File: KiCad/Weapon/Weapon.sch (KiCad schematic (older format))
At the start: 29 parts, among them IC1 ATMEGA328-P, J1 MICRO_USB, P1 2P_CGRID_M, P2 USB-TTL, P3 2P_CGRID_M, Q1 NPN, U1 MCP73831, U2 RFID-RC522, U3 LM1084IT-3.3/NOPB, X1 16MHz

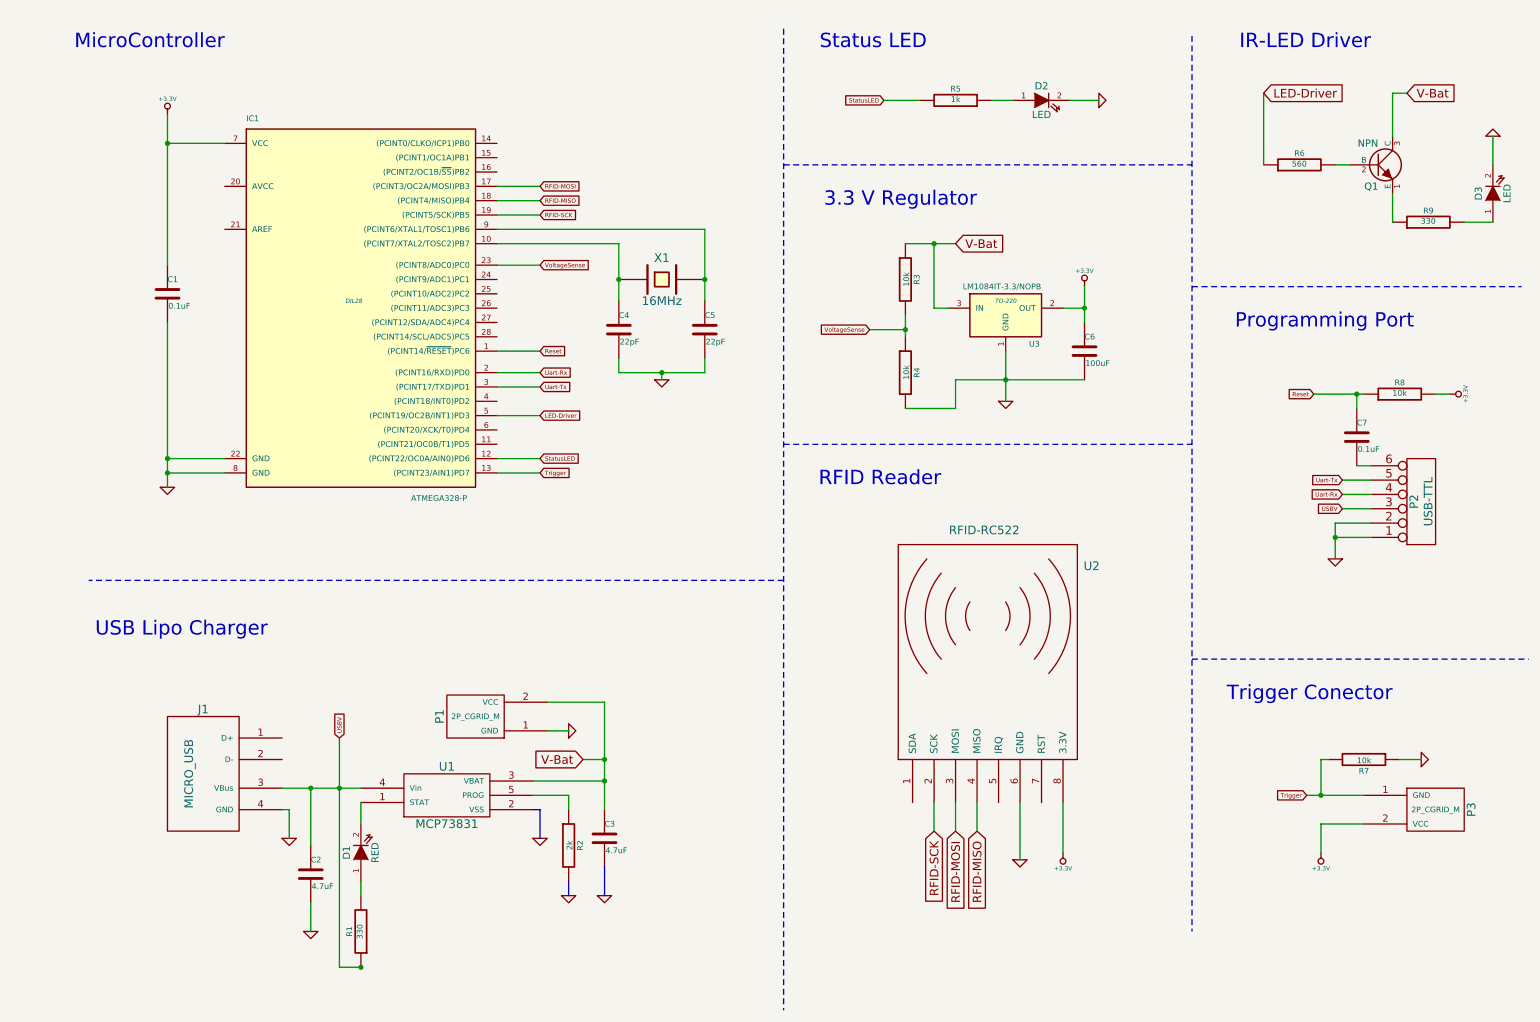
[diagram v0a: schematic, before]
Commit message: Revert "Revert "3/29 KiCad Updates""
This reverts commit 46467126b97e8d3ee2ff82587e11af580e6d6854.
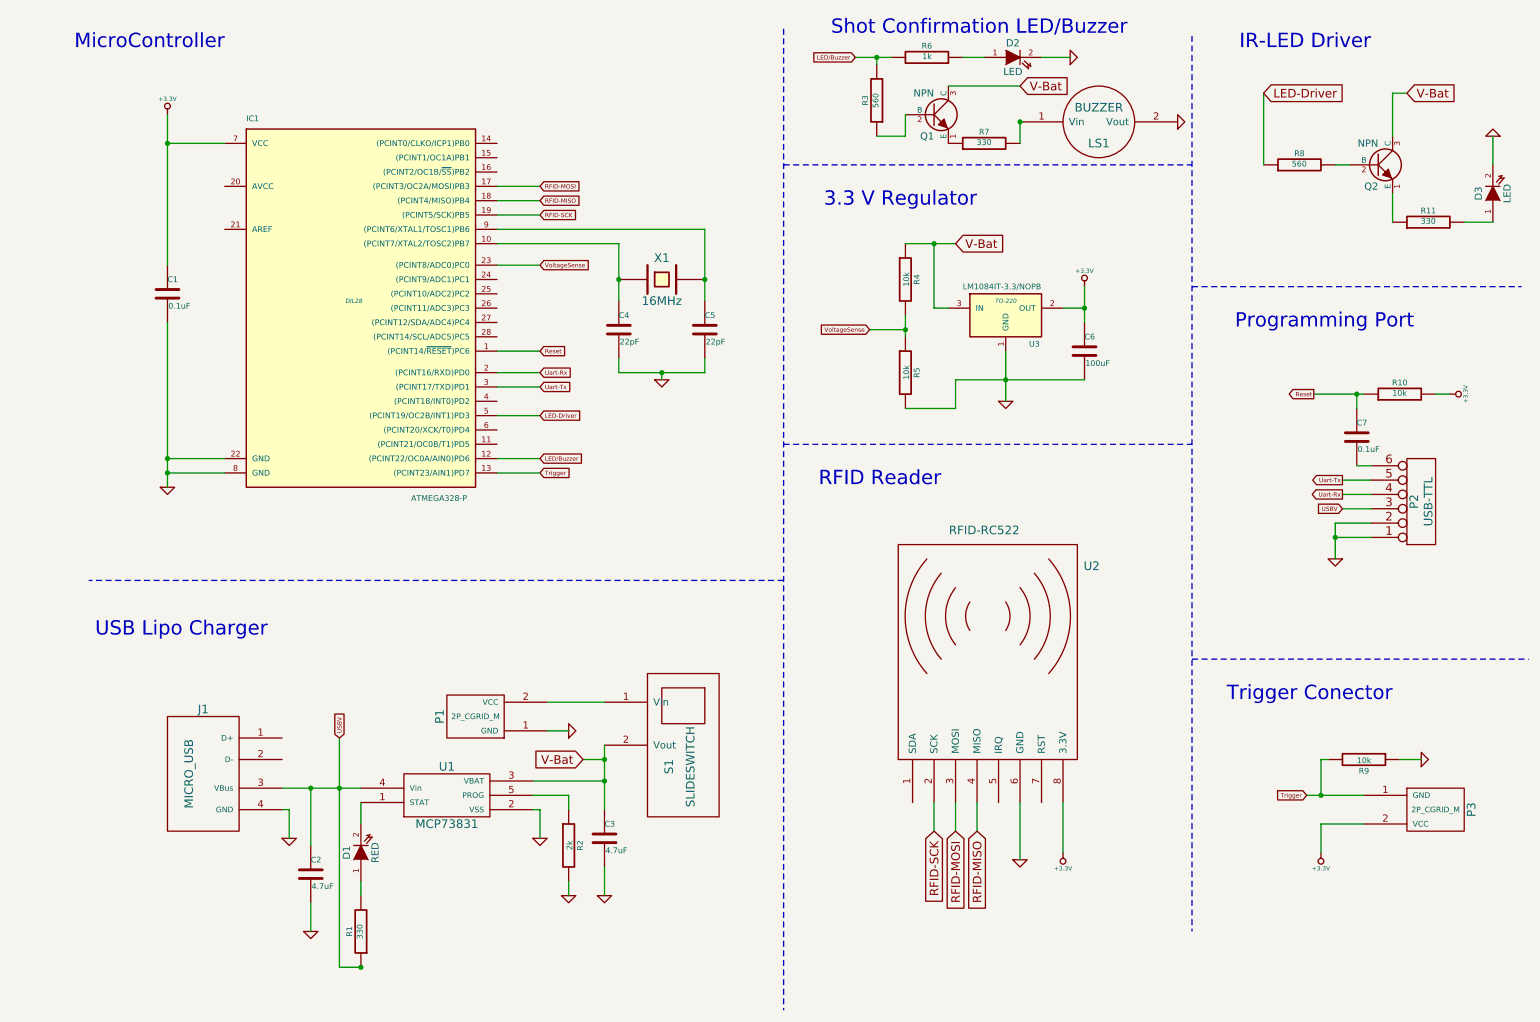
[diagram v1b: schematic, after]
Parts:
- added LS1: BUZZER, symbol BUZZER
- added Q1: NPN, ~, symbol NPN
- added R3: 560, ~, symbol R
- added R7: 330, ~, symbol R
- added S1: SLIDESWITCH, symbol SLIDESWITCH
- renumbered Q1 to Q2, R8 to R10, R9 to R11, R3 to R4, R4 to R5, R5 to R6, R6 to R8, R7 to R9
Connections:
- net GND: now also C3.2, R2.2, U1.2 (VSS), LS1.2 (Vout)
- net V-Bat: now also Q1.3 (C), S1.2 (Vout); no longer P1.2 (VCC)
- net StatusLED renamed LED/Buzzer
- net LED/Buzzer: now also R3.2
- new net: P1.2 (VCC), S1.1 (Vin)
- new net: Q1.1 (E), R7.1
- new net: Q1.2 (B), R3.1
- new net: LS1.1 (Vin), R7.2
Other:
- note added: "Shot Confirmation LED/Buzzer"
- note removed: "Status LED\n"
- moved on the sheet: D2, R6

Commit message: Revert "3/29 KiCad Updates"
This reverts commit a2529da1b40b1f6e0e832ed1976ed3be41434859.
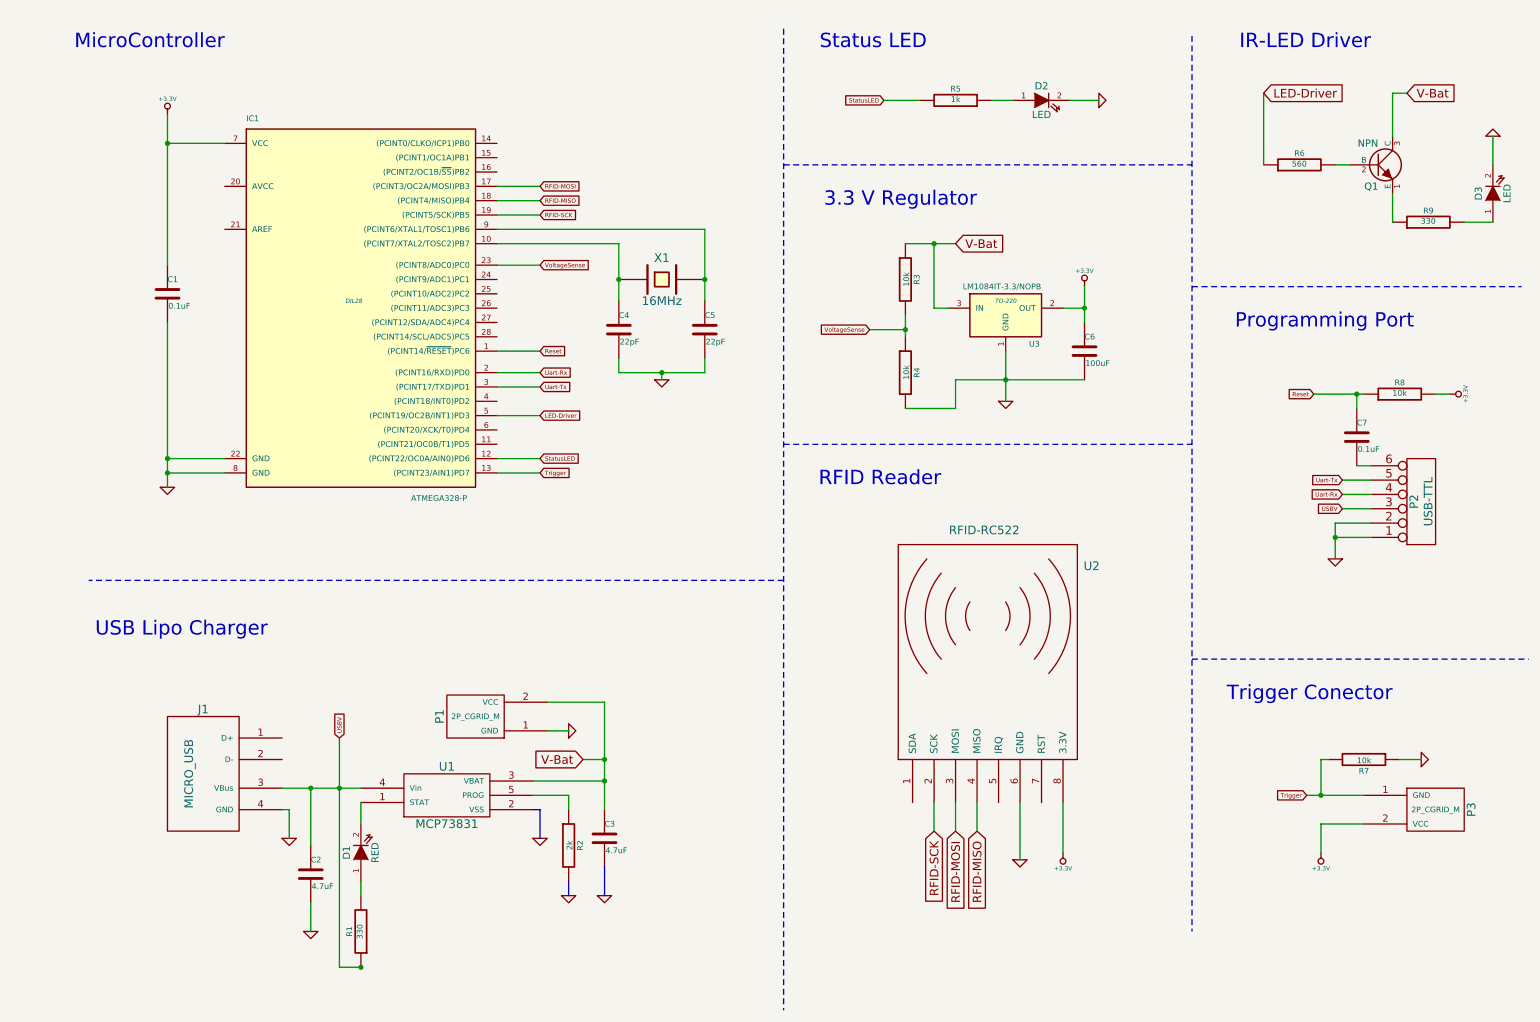
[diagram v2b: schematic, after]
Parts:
- removed LS1: BUZZER, symbol BUZZER
- removed Q1: NPN, ~, symbol NPN
- removed R3: 560, ~, symbol R
- removed R7: 330, ~, symbol R
- removed S1: SLIDESWITCH, symbol SLIDESWITCH
- renumbered Q2 to Q1, R4 to R3, R5 to R4, R6 to R5, R8 to R6, R9 to R7, R10 to R8, R11 to R9
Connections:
- net GND: no longer C3.2, R2.2, U1.2 (VSS)
- net V-Bat: now also P1.2 (VCC)
- net LED/Buzzer renamed StatusLED
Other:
- note added: "Status LED\n"
- note removed: "Shot Confirmation LED/Buzzer"
- moved on the sheet: D2, R5
